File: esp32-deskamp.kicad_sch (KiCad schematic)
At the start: 29 parts, among them J1 INPUT 00, J10 ADDITIONAL GPIO, J2 INPUT 01, J3 MUTE, J4 SLEEP, J5 PRE OUT, J6 LFE OUT, J7 INPUT SELECT, J8 MOTOR, J9 12V IN, K1 INPUT 00, K2 INPUT 01, K3 AMP MUTE, K4 AMP SLEEP, U1 ESP32 D1 MINI, U2 TSR 1-2433, U3 L9110, U4 ULN2003A

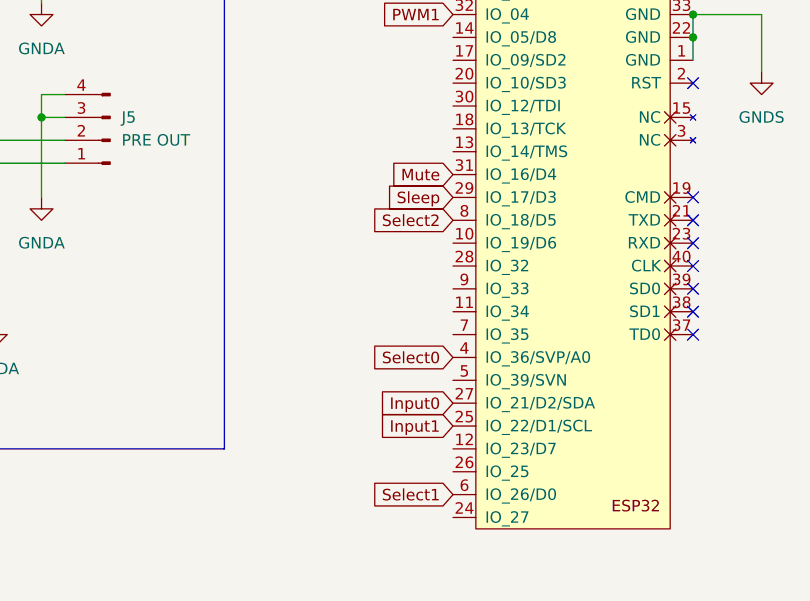
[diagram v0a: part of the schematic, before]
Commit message: IC routing
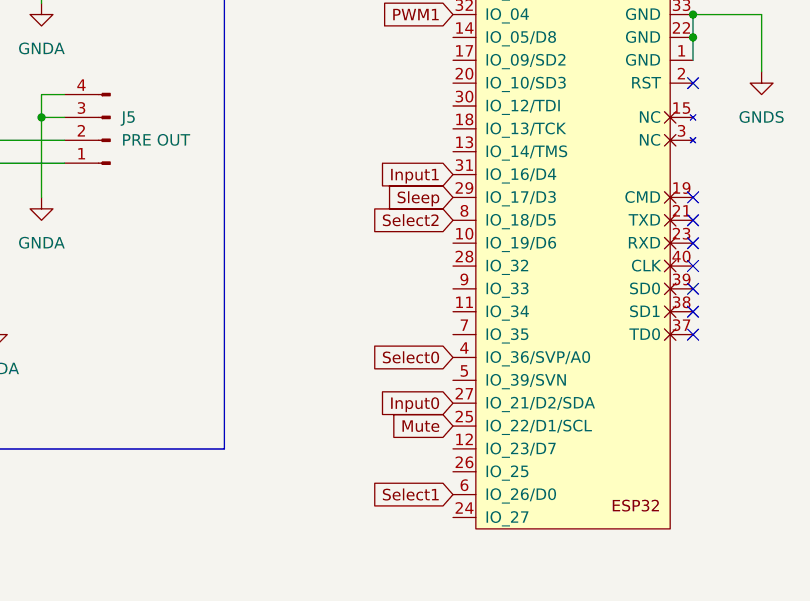
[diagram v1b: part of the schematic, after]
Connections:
- net Input1: now also U1.31 (IO_16/D4); no longer U1.25 (IO_22/D1/SCL)
- net Mute: now also U1.25 (IO_22/D1/SCL); no longer U1.31 (IO_16/D4)

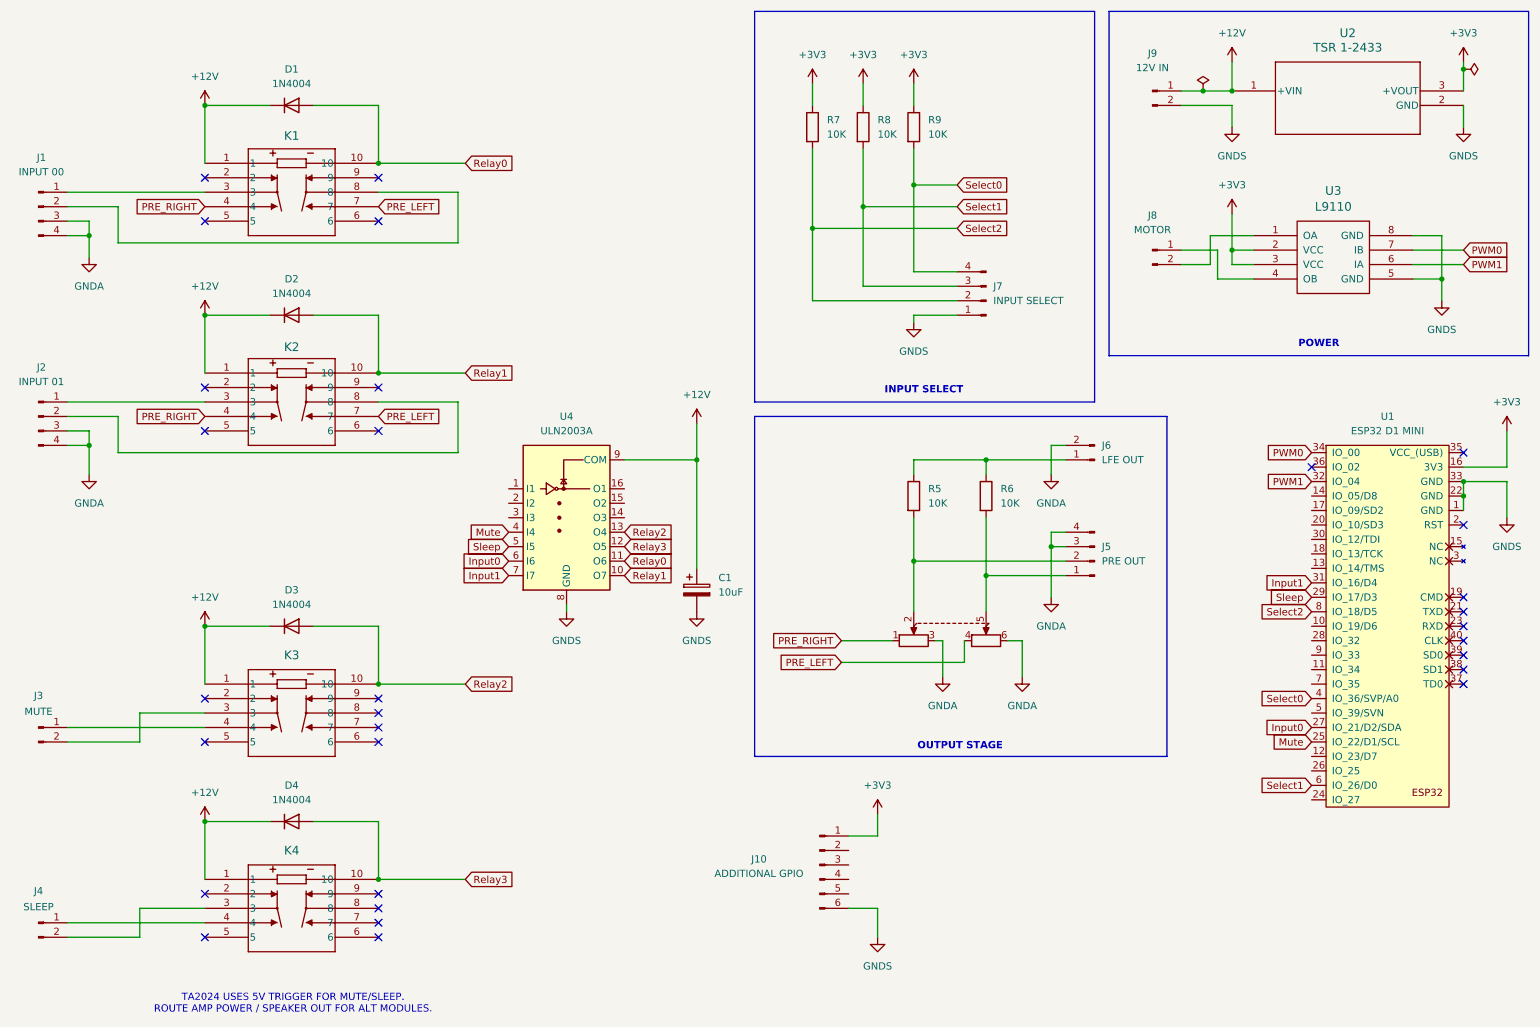
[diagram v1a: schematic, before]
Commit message: IC routing
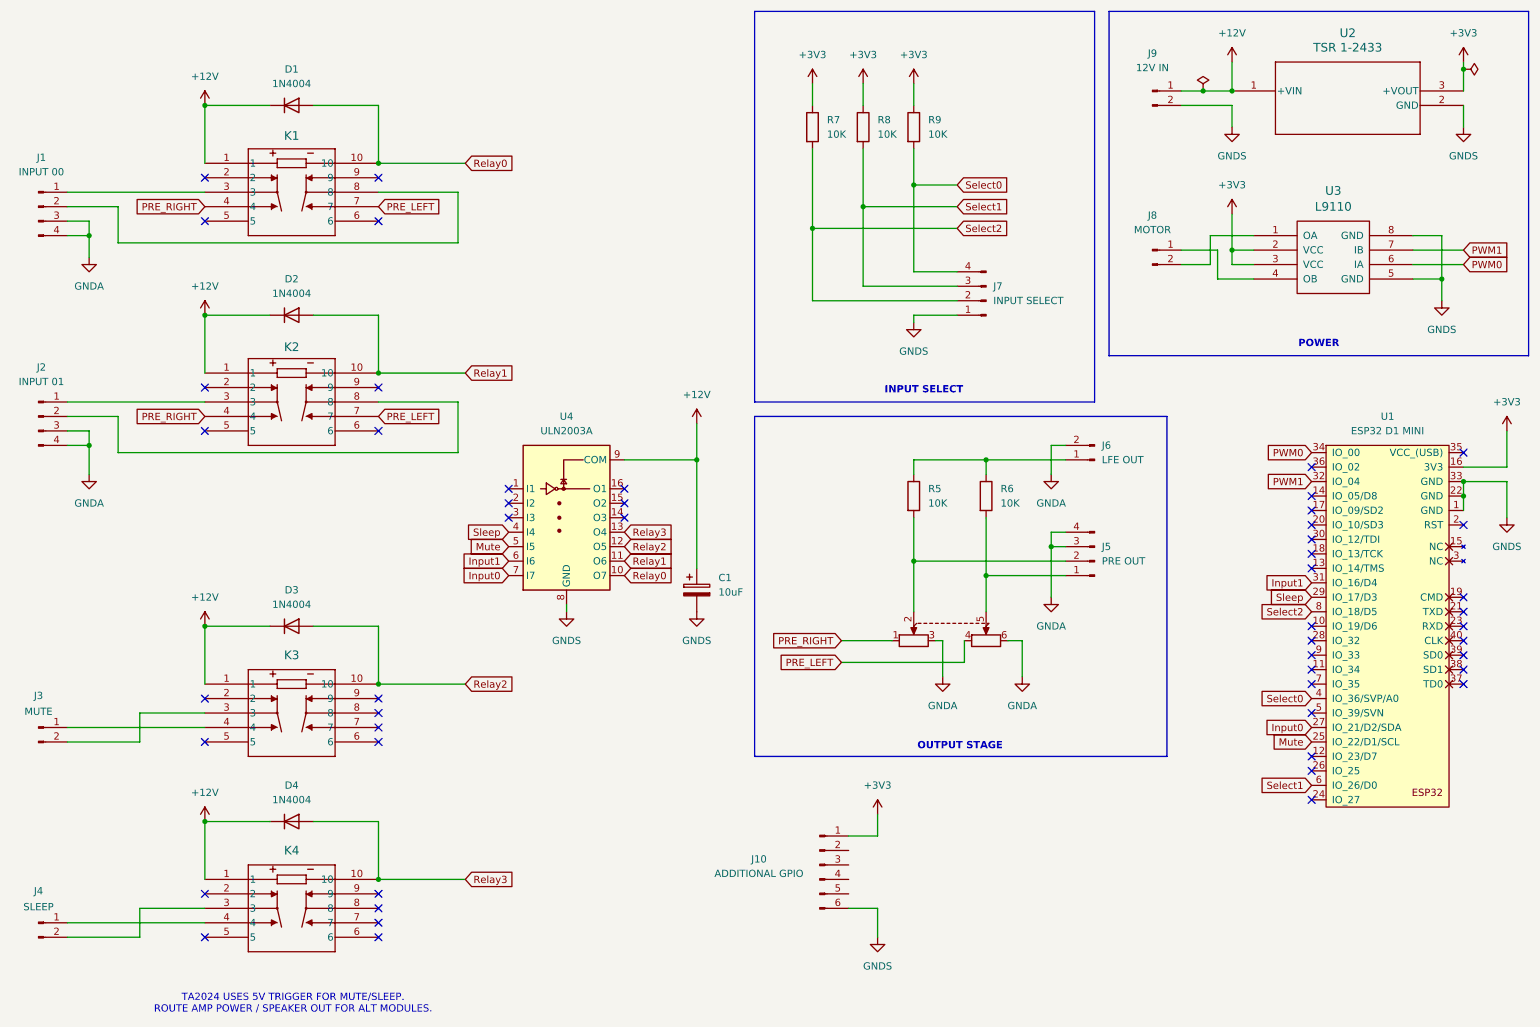
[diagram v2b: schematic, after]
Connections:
- net Input0: now also U4.7 (I7); no longer U4.6 (I6)
- net Input1: now also U4.6 (I6); no longer U4.7 (I7)
- net Mute: now also U4.5 (I5); no longer U4.4 (I4)
- net PWM0: now also U3.6 (IA); no longer U3.7 (IB)
- net PWM1: now also U3.7 (IB); no longer U3.6 (IA)
- net Relay0: now also U4.10 (O7); no longer U4.11 (O6)
- net Relay1: now also U4.11 (O6); no longer U4.10 (O7)
- net Relay2: now also U4.12 (O5); no longer U4.13 (O4)
- net Relay3: now also U4.13 (O4); no longer U4.12 (O5)
- net Sleep: now also U4.4 (I4); no longer U4.5 (I5)
- no-connect marks 30 -> 51
